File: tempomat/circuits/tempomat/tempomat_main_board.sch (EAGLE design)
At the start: 59 parts, among them Q1 2N4033, Q2 BC489, T1 TIP122, T2 TIP32C, T2-TIP127 BDX54, T3 TIP122, T4-TIP127 BDX54, U2 LM747N, U4_XOR- 4070N, U5-LM2931 78L05Z

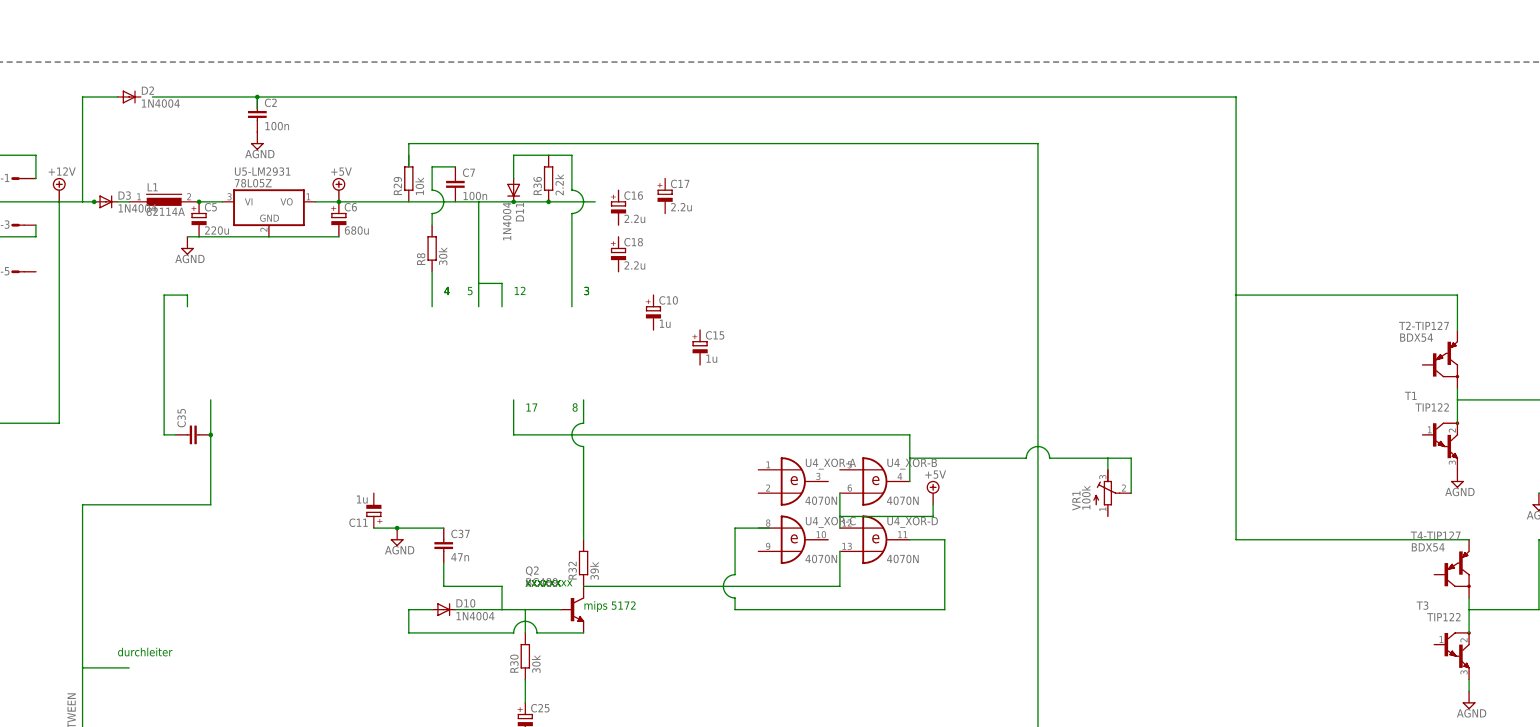
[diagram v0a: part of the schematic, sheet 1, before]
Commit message: reg save
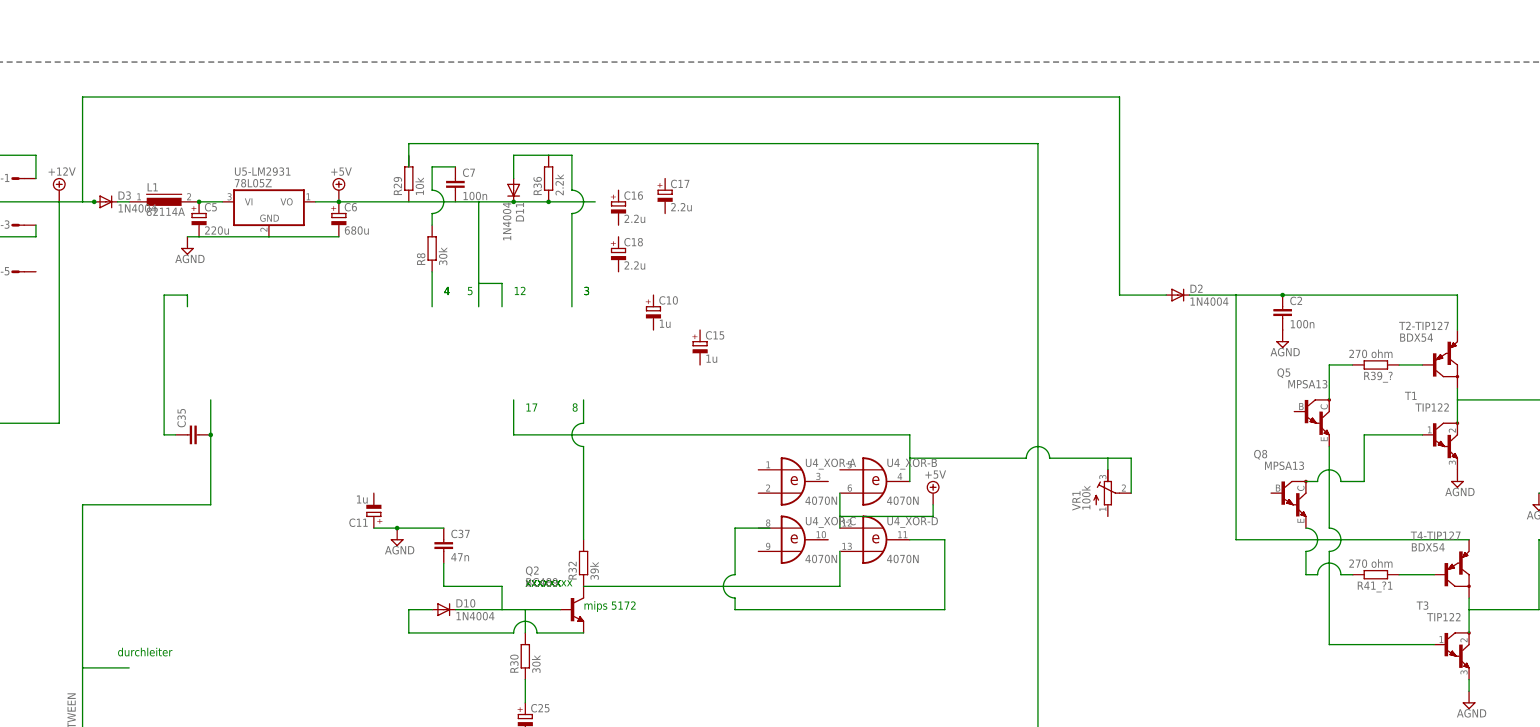
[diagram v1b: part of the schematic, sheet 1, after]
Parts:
- added Q5, Q8: MPSA13, transistor:MMBTA13LT1-NPN_DARL-SOT23-BEC
- added R39_?, R41_?1: 270 ohm, resistor:R-EU_0204/2V
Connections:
- new net N$4: R39_?.1, T2-TIP127.B
- new net N$40: Q5.C, R39_?.2
- new net N$41: Q5.E, T3.B
- new net N$42: R41_?1.1, T4-TIP127.B
- new net N$43: Q8.E, R41_?1.2
- new net N$44: Q8.C, T1.B
- net N$31: now also D2.C
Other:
- moved on the sheet: C2, D2
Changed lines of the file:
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@@
 <part name="R1" library="resistor" deviceset="R-EU_" device="0204/2V" value="7.4k"/>
 <part name="SUPPLY16" library="supply2" deviceset="AGND" device=""/>
+<part name="R39_?" library="resistor" deviceset="R-EU_" device="0204/2V" value="270 ohm"/>
+<part name="Q5" library="transistor" deviceset="*-NPN_DARL-" device="SOT23-BEC" technology="MMBTA13LT1" value="MPSA13"/>
+<part name="R41_?1" library="resistor" deviceset="R-EU_" device="0204/2V" value="270 ohm"/>
+<part name="Q8" library="transistor" deviceset="*-NPN_DARL-" device="SOT23-BEC" technology="MMBTA13LT1" value="MPSA13"/>
 </parts>
 <sheets>
@@
 <instance part="C1" gate="G$1" x="-7.62" y="30.48"/>
 <instance part="SUPPLY3" gate="+12V" x="30.48" y="93.98"/>
-<instance part="D2" gate="1" x="45.72" y="114.3"/>
+<instance part="D2" gate="1" x="274.32" y="71.12"/>
 <instance part="C16" gate="G$1" x="152.4" y="91.44"/>
 <instance part="C17" gate="G$1" x="162.56" y="93.98"/>
@@
 <instance part="VR1" gate="G$1" x="259.08" y="27.94"/>
 <instance part="J_ACTUATOR" gate="G$1" x="370.84" y="17.78"/>
-<instance part="C2" gate="G$1" x="73.66" y="111.76"/>
-<instance part="SUPPLY10" gate="G$1" x="73.66" y="104.14"/>
+<instance part="C2" gate="G$1" x="297.18" y="68.58"/>
+<instance part="SUPPLY10" gate="G$1" x="297.18" y="60.96"/>
 <instance part="SUPPLY12" gate="G$1" x="337.82" y="-17.78"/>
 <instance part="SUPPLY13" gate="G$1" x="335.28" y="30.48"/>
@@
 <instance part="R1" gate="G$1" x="381" y="78.74" rot="R180"/>
 <instance part="SUPPLY16" gate="G$1" x="104.14" y="17.78"/>
+<instance part="R39_?" gate="G$1" x="317.5" y="55.88" rot="R180"/>
+<instance part="Q5" gate="G$1" x="302.26" y="45.72"/>
+<instance part="R41_?1" gate="G$1" x="317.5" y="10.16" rot="R180"/>
+<instance part="Q8" gate="G$1" x="297.18" y="27.94"/>
 </instances>
 <busses>
@@
 <wire x1="30.48" y1="91.44" x2="35.56" y2="91.44" width="0.1524" layer="91"/>
 <wire x1="35.56" y1="91.44" x2="35.56" y2="114.3" width="0.1524" layer="91"/>
+<wire x1="35.56" y1="114.3" x2="261.62" y2="114.3" width="0.1524" layer="91"/>
+<wire x1="261.62" y1="114.3" x2="261.62" y2="71.12" width="0.1524" layer="91"/>
 <pinref part="D2" gate="1" pin="A"/>
-<wire x1="35.56" y1="114.3" x2="43.18" y2="114.3" width="0.1524" layer="91"/>
+<wire x1="261.62" y1="71.12" x2="271.78" y2="71.12" width="0.1524" layer="91"/>
 </segment>
 </net>
@@
 <net name="N$31" class="0">
 <segment>
-<wire x1="50.8" y1="114.3" x2="73.66" y2="114.3" width="0.1524" layer="91"/>
-<wire x1="73.66" y1="114.3" x2="73.66" y2="111.76" width="0.1524" layer="91"/>
-<pinref part="C2" gate="G$1" pin="1"/>
-<junction x="73.66" y="114.3"/>
-<wire x1="73.66" y1="114.3" x2="287.02" y2="114.3" width="0.1524" layer="91"/>
-<wire x1="287.02" y1="114.3" x2="287.02" y2="71.12" width="0.1524" layer="91"/>
-<wire x1="287.02" y1="71.12" x2="335.28" y2="71.12" width="0.1524" layer="91"/>
+<wire x1="287.02" y1="71.12" x2="297.18" y2="71.12" width="0.1524" layer="91"/>
 <pinref part="T2-TIP127" gate="G$1" pin="E"/>
+<wire x1="297.18" y1="71.12" x2="335.28" y2="71.12" width="0.1524" layer="91"/>
 <wire x1="335.28" y1="71.12" x2="335.28" y2="63.5" width="0.1524" layer="91"/>
 <wire x1="287.02" y1="71.12" x2="287.02" y2="17.78" width="0.1524" layer="91"/>
 <pinref part="T4-TIP127" gate="G$1" pin="E"/>
 <wire x1="287.02" y1="17.78" x2="337.82" y2="17.78" width="0.1524" layer="91"/>
+<pinref part="C2" gate="G$1" pin="1"/>
+<junction x="297.18" y="71.12"/>
+<pinref part="D2" gate="1" pin="C"/>
+<wire x1="276.86" y1="71.12" x2="287.02" y2="71.12" width="0.1524" layer="91"/>
 </segment>
 </net>
@@
 </segment>
 </net>
+<net name="N$4" class="0">
+<segment>
+<pinref part="R39_?" gate="G$1" pin="1"/>
+<pinref part="T2-TIP127" gate="G$1" pin="B"/>
+<wire x1="322.58" y1="55.88" x2="327.66" y2="55.88" width="0.1524" layer="91"/>
+</segment>
+</net>
+<net name="N$40" class="0">
+<segment>
+<pinref part="R39_?" gate="G$1" pin="2"/>
+<wire x1="312.42" y1="55.88" x2="307.34" y2="55.88" width="0.1524" layer="91"/>
+<pinref part="Q5" gate="G$1" pin="C"/>
+<wire x1="307.34" y1="55.88" x2="307.34" y2="48.26" width="0.1524" layer="91"/>
+</segment>
+</net>
+<net name="N$41" class="0">
+<segment>
+<pinref part="Q5" gate="G$1" pin="E"/>
+<wire x1="307.34" y1="38.1" x2="307.34" y2="20.32" width="0.1524" layer="91"/>
+<wire x1="307.34" y1="20.32" x2="307.34" y2="15.24" width="0.1524" layer="91" curve="-180"/>
+<wire x1="307.34" y1="15.24" x2="307.34" y2="-5.08" width="0.1524" layer="91"/>
+<pinref part="T3" gate="G$1" pin="B"/>
+<wire x1="307.34" y1="-5.08" x2="330.2" y2="-5.08" width="0.1524" layer="91"/>
+</segment>
+</net>
+<net name="N$42" class="0">
+<segment>
+<pinref part="R41_?1" gate="G$1" pin="1"/>
+<pinref part="T4-TIP127" gate="G$1" pin="B"/>
+<wire x1="322.58" y1="10.16" x2="330.2" y2="10.16" width="0.1524" layer="91"/>
+</segment>
+</net>
+<net name="N$43" class="0">
+<segment>
+<pinref part="Q8" gate="G$1" pin="E"/>
+<wire x1="302.26" y1="20.32" x2="302.26" y2="15.24" width="0.1524" layer="91" curve="-180"/>
+<wire x1="302.26" y1="15.24" x2="302.26" y2="10.16" width="0.1524" layer="91"/>
+<wire x1="302.26" y1="10.16" x2="304.8" y2="10.16" width="0.1524" layer="91"/>
+<wire x1="304.8" y1="10.16" x2="309.88" y2="10.16" width="0.1524" layer="91" curve="-180"/>
+<pinref part="R41_?1" gate="G$1" pin="2"/>
+<wire x1="309.88" y1="10.16" x2="312.42" y2="10.16" width="0.1524" layer="91"/>
+</segment>
+</net>
+<net name="N$44" class="0">
+<segment>
+<pinref part="Q8" gate="G$1" pin="C"/>
+<wire x1="302.26" y1="30.48" x2="304.8" y2="30.48" width="0.1524" layer="91"/>
+<wire x1="304.8" y1="30.48" x2="309.88" y2="30.48" width="0.1524" layer="91" curve="-180"/>
+<wire x1="309.88" y1="30.48" x2="314.96" y2="30.48" width="0.1524" layer="91"/>
+<wire x1="314.96" y1="30.48" x2="314.96" y2="40.64" width="0.1524" layer="91"/>
+<pinref part="T1" gate="G$1" pin="B"/>
+<wire x1="314.96" y1="40.64" x2="327.66" y2="40.64" width="0.1524" layer="91"/>
+</segment>
+</net>

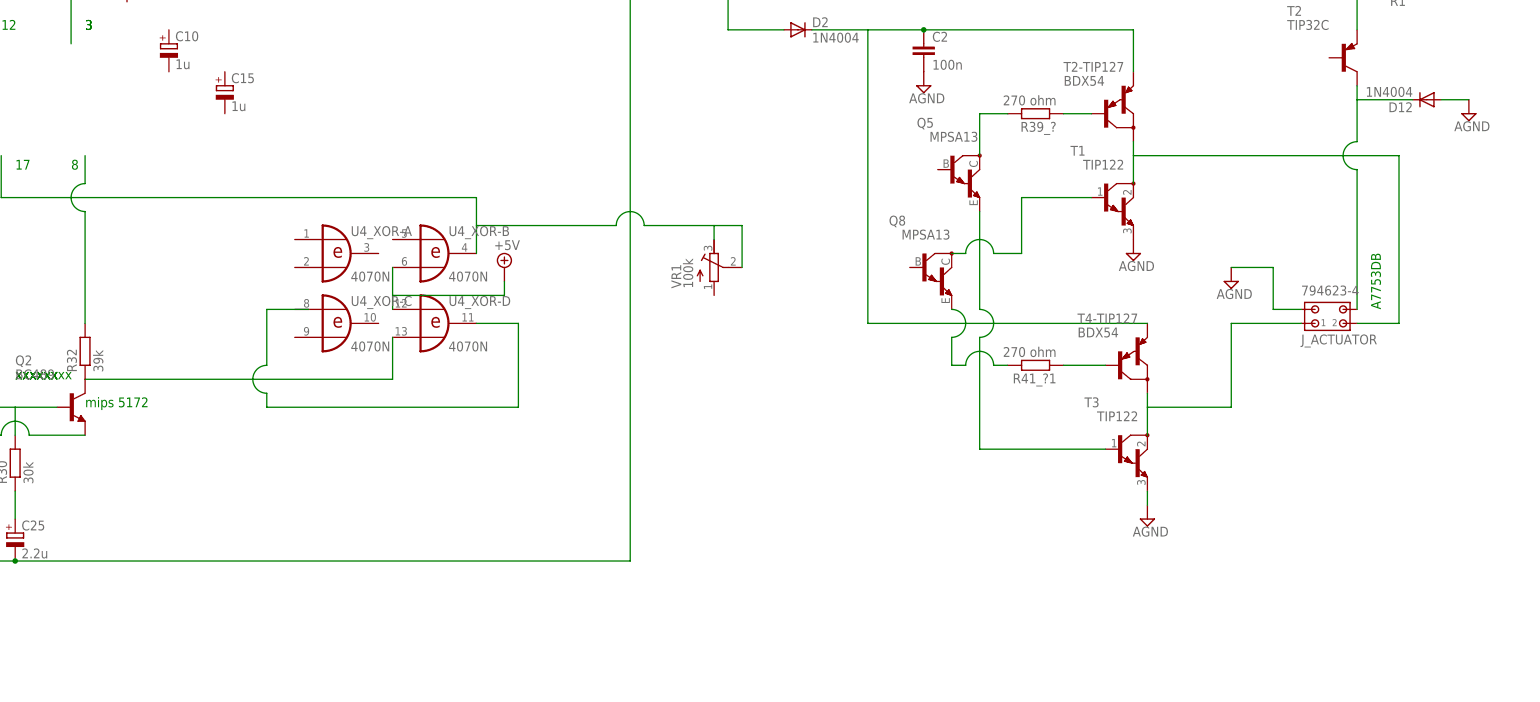
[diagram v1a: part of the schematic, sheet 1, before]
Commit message: reg save
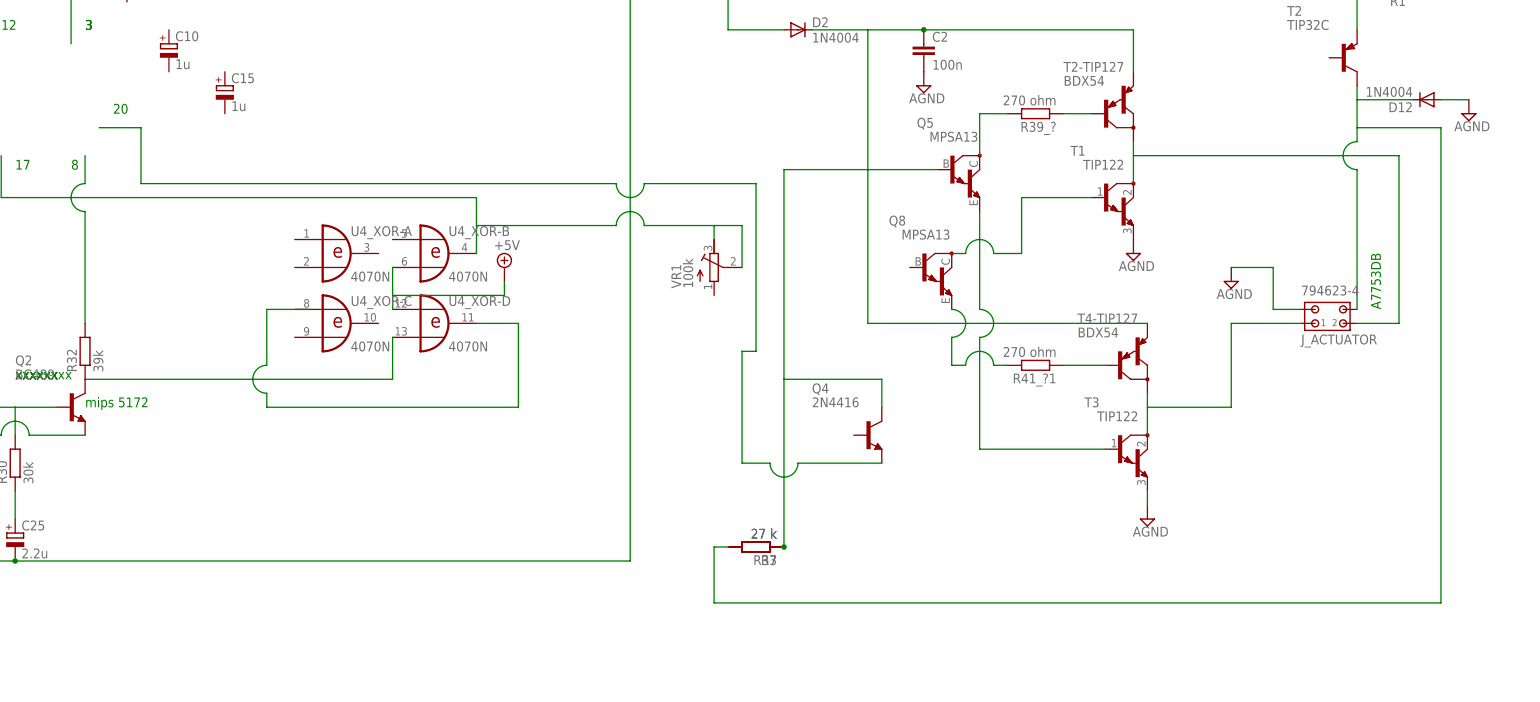
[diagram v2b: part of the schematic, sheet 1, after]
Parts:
- added Q4: 2N4416, transistor-npn:2N4416
- added R3, R37: 27 k, resistor:R-EU_0204/2V
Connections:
- new net N$45: Q4.C, Q5.B, R3.1, R37.1
- new net N$46: D12.C, J_ACTUATOR.4, R3.2, R37.2, T2.C
- net N$36: now also Q4.E; no longer D12.C, J_ACTUATOR.4, T2.C
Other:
- note added: "20"
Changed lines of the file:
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@@
 <part name="R41_?1" library="resistor" deviceset="R-EU_" device="0204/2V" value="270 ohm"/>
 <part name="Q8" library="transistor" deviceset="*-NPN_DARL-" device="SOT23-BEC" technology="MMBTA13LT1" value="MPSA13"/>
+<part name="R37" library="resistor" deviceset="R-EU_" device="0204/2V" value="27 k"/>
+<part name="R3" library="resistor" deviceset="R-EU_" device="0204/2V" value="27 k"/>
+<part name="Q4" library="transistor-npn" deviceset="2N4416" device=""/>
 </parts>
 <sheets>
@@
 <text x="381" y="116.84" size="1.778" layer="91">12V if hmi ON</text>
 <text x="142.24" y="45.72" size="1.778" layer="91">8</text>
+<text x="149.86" y="55.88" size="1.778" layer="91">20</text>
 </plain>
 <instances>
@@
 <instance part="R41_?1" gate="G$1" x="317.5" y="10.16" rot="R180"/>
 <instance part="Q8" gate="G$1" x="297.18" y="27.94"/>
+<instance part="R37" gate="G$1" x="266.7" y="-22.86" rot="R180"/>
+<instance part="R3" gate="G$1" x="266.7" y="-22.86" rot="R180"/>
+<instance part="Q4" gate="G$1" x="287.02" y="-2.54"/>
 </instances>
 <busses>
@@
 </segment>
 </net>
-<net name="N$36" class="0">
-<segment>
-<pinref part="J_ACTUATOR" gate="G$1" pin="4"/>
-<wire x1="375.92" y1="20.32" x2="375.92" y2="45.72" width="0.1524" layer="91"/>
-<wire x1="375.92" y1="45.72" x2="375.92" y2="50.8" width="0.1524" layer="91" curve="-180"/>
-<wire x1="375.92" y1="50.8" x2="375.92" y2="58.42" width="0.1524" layer="91"/>
-<pinref part="T2" gate="G$1" pin="C"/>
-<pinref part="D12" gate="1" pin="C"/>
-<wire x1="375.92" y1="58.42" x2="375.92" y2="60.96" width="0.1524" layer="91"/>
-<wire x1="375.92" y1="58.42" x2="386.08" y2="58.42" width="0.1524" layer="91"/>
-</segment>
-</net>
 <net name="N$33" class="0">
 <segment>
@@
 </segment>
 </net>
+<net name="N$45" class="0">
+<segment>
+<pinref part="Q5" gate="G$1" pin="B"/>
+<wire x1="299.72" y1="45.72" x2="271.78" y2="45.72" width="0.1524" layer="91"/>
+<wire x1="271.78" y1="45.72" x2="271.78" y2="7.62" width="0.1524" layer="91"/>
+<pinref part="R37" gate="G$1" pin="1"/>
+<junction x="271.78" y="-22.86"/>
+<pinref part="R3" gate="G$1" pin="1"/>
+<wire x1="271.78" y1="7.62" x2="271.78" y2="-22.86" width="0.1524" layer="91"/>
+<wire x1="271.78" y1="7.62" x2="289.56" y2="7.62" width="0.1524" layer="91"/>
+<pinref part="Q4" gate="G$1" pin="C"/>
+<wire x1="289.56" y1="7.62" x2="289.56" y2="2.54" width="0.1524" layer="91"/>
+</segment>
+</net>
+<net name="N$46" class="0">
+<segment>
+<pinref part="R37" gate="G$1" pin="2"/>
+<pinref part="R3" gate="G$1" pin="2"/>
+<wire x1="261.62" y1="-22.86" x2="259.08" y2="-22.86" width="0.1524" layer="91"/>
+<wire x1="259.08" y1="-22.86" x2="259.08" y2="-33.02" width="0.1524" layer="91"/>
+<wire x1="259.08" y1="-33.02" x2="391.16" y2="-33.02" width="0.1524" layer="91"/>
+<wire x1="391.16" y1="-33.02" x2="391.16" y2="53.34" width="0.1524" layer="91"/>
+<pinref part="J_ACTUATOR" gate="G$1" pin="4"/>
+<wire x1="375.92" y1="20.32" x2="375.92" y2="45.72" width="0.1524" layer="91"/>
+<wire x1="375.92" y1="45.72" x2="375.92" y2="50.8" width="0.1524" layer="91" curve="-180"/>
+<wire x1="375.92" y1="50.8" x2="375.92" y2="53.34" width="0.1524" layer="91"/>
+<pinref part="T2" gate="G$1" pin="C"/>
+<pinref part="D12" gate="1" pin="C"/>
+<wire x1="375.92" y1="53.34" x2="375.92" y2="58.42" width="0.1524" layer="91"/>
+<wire x1="375.92" y1="58.42" x2="375.92" y2="60.96" width="0.1524" layer="91"/>
+<wire x1="375.92" y1="58.42" x2="386.08" y2="58.42" width="0.1524" layer="91"/>
+<wire x1="391.16" y1="53.34" x2="375.92" y2="53.34" width="0.1524" layer="91"/>
+</segment>
+</net>
+<net name="N$36" class="0">
+<segment>
+<pinref part="Q4" gate="G$1" pin="E"/>
+<wire x1="289.56" y1="-7.62" x2="274.32" y2="-7.62" width="0.1524" layer="91"/>
+<wire x1="274.32" y1="-7.62" x2="269.24" y2="-7.62" width="0.1524" layer="91" curve="-180"/>
+<wire x1="269.24" y1="-7.62" x2="264.16" y2="-7.62" width="0.1524" layer="91"/>
+<wire x1="264.16" y1="-7.62" x2="264.16" y2="12.7" width="0.1524" layer="91"/>
+<wire x1="264.16" y1="12.7" x2="266.7" y2="12.7" width="0.1524" layer="91"/>
+<wire x1="266.7" y1="12.7" x2="266.7" y2="43.18" width="0.1524" layer="91"/>
+<wire x1="266.7" y1="43.18" x2="246.38" y2="43.18" width="0.1524" layer="91"/>
+<wire x1="246.38" y1="43.18" x2="241.3" y2="43.18" width="0.1524" layer="91" curve="-180"/>
+<wire x1="241.3" y1="43.18" x2="154.94" y2="43.18" width="0.1524" layer="91"/>
+<wire x1="154.94" y1="43.18" x2="154.94" y2="53.34" width="0.1524" layer="91"/>
+<wire x1="154.94" y1="53.34" x2="147.32" y2="53.34" width="0.1524" layer="91"/>
+</segment>
+</net>
